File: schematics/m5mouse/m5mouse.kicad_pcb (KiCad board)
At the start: 2 copper layers, 110 x 50 mm, 98 parts, among them IC1 LM3940IMP-3.3_NOPB, J1 Conn_01x02, J2 M-BUS, J3 SWD, J4 Conn_02x03_Odd_Even, J5 Conn_02x03_Odd_Even, J6 Conn_01x03, J7 Conn_01x06, J8 Conn_01x06, Q1 BSS138, Q2 ST-1KL3A, Q3 BSS138, Q4 ST-1KL3A, Q5 BSS138, Q6 ST-1KL3A, Q7 BSS138, Q8 ST-1KL3A, SW1 SW_SPDT, SW2 SW_Push, U1 TPS562200, U2 STM32F405RGTx, U3 DRV8835, U4 MPU9250_9255, Y1 8MHz, Y2 32.768kHz

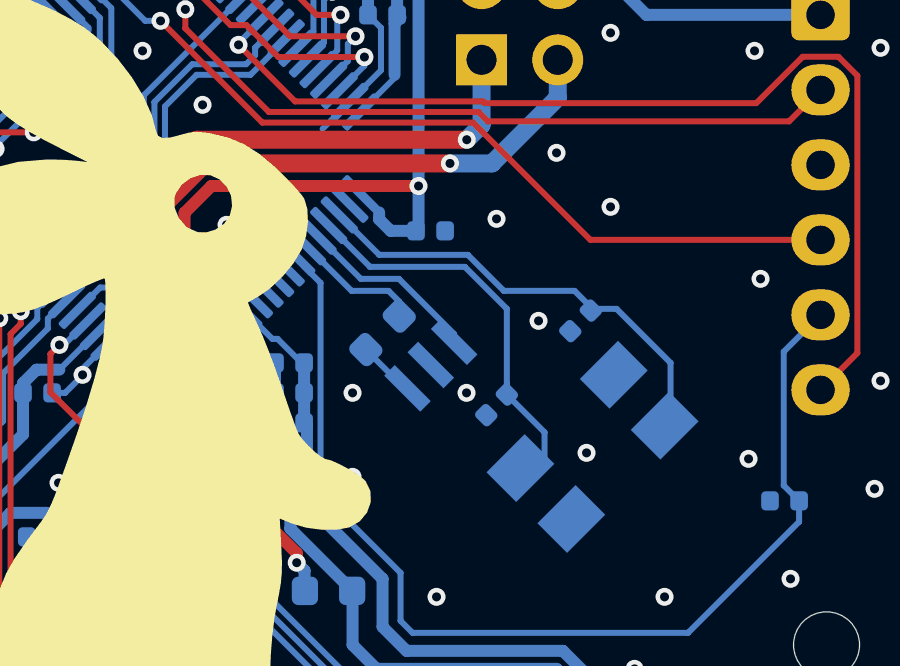
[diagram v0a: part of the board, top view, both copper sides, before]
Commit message: Fix pattern
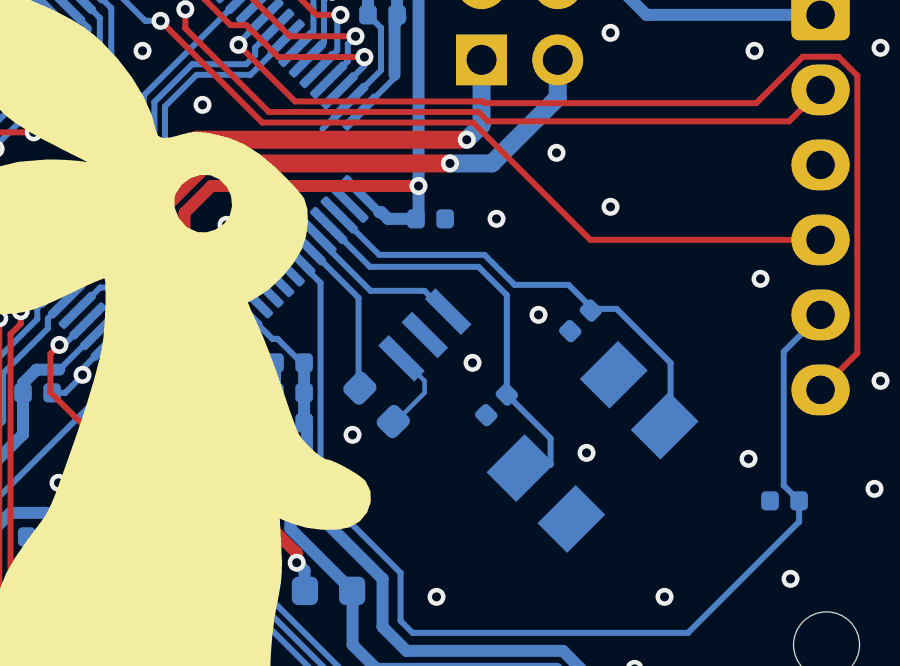
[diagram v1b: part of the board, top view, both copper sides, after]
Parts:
- moved R4 2.41 mm to (172.2, 112.0), turned to 315 degrees
- moved Y1 1.02 mm to (175.4, 109.0)
- moved C28 0.40 mm to (174.0, 105.8)
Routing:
- net Net-(R4-Pad1): track 4.30 -> 5.38 mm
- net Net-(R4-Pad2): track 1.92 -> 2.95 mm
- net +3V3: track 189.7 -> 189.0 mm
- net Net-(C9-Pad1): track 13.2 -> 13.8 mm
- net Net-(U2-Pad5): track 6.14 -> 5.48 mm
- net GND: vias 136 -> 135
